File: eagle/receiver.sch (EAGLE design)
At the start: 20 parts, among them IC1 7805T, U1 ARDUINOR3-DIMENSION

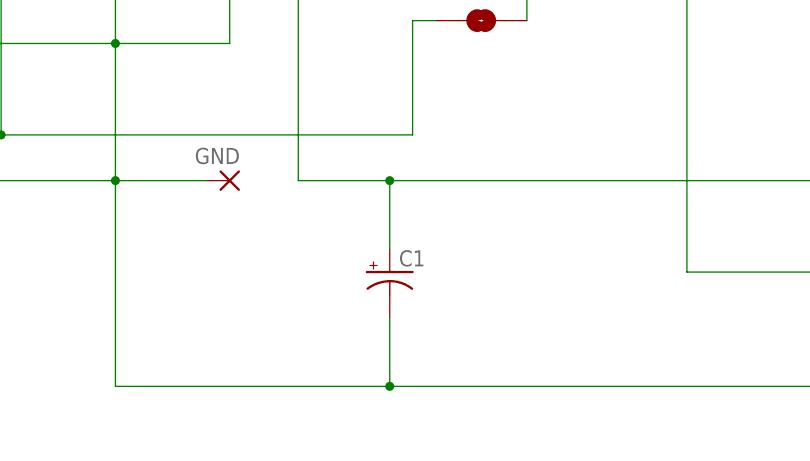
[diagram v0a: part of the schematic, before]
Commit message: Docs++
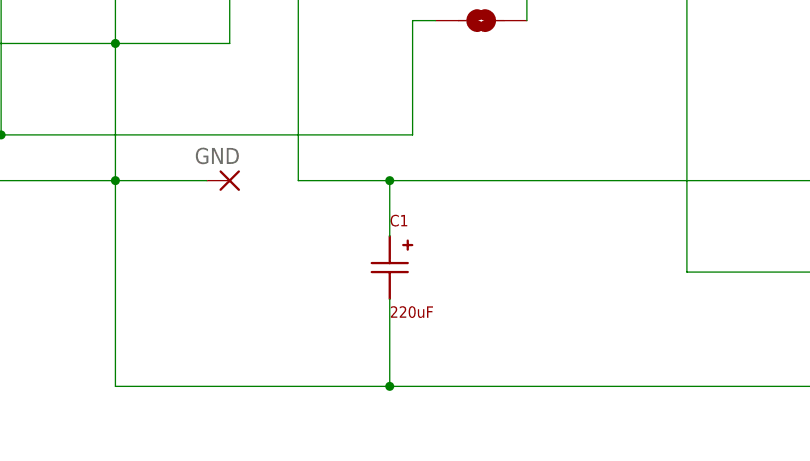
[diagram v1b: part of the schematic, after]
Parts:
- C1: value (none) -> 220uF; device adafruit:CPOL-US153CLV-0405 -> phrobo:UWT0J221MCL1GB
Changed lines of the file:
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@@
 <part name="RESET" library="SparkFun" deviceset="TAC_SWITCH" device="SMD"/>
 <part name="JP7" library="SparkFun" deviceset="M02" device="PTH"/>
-<part name="C1" library="adafruit" deviceset="CPOL-US" device="153CLV-0405"/>
+<part name="C1" library="phrobo" deviceset="UWT0J221MCL1GB" device="" value="220uF"/>
 <part name="D1" library="adafruit" deviceset="DIODE" device="SMA"/>
 <part name="VCC/+5V" library="SparkFun" deviceset="SOLDERJUMPER" device="NO" value="NC=+5v"/>
@@
 <junction x="45.72" y="86.36"/>
 <pinref part="C1" gate="G$1" pin="-"/>
-<wire x1="63.5" y1="20.32" x2="63.5" y2="12.7" width="0.1524" layer="91"/>
+<wire x1="63.5" y1="22.4" x2="63.5" y2="12.7" width="0.1524" layer="91"/>
 <junction x="63.5" y="12.7"/>
 </segment>
@@
 <wire x1="53.34" y1="88.9" x2="101.6" y2="88.9" width="0.1524" layer="91"/>
 <pinref part="C1" gate="G$1" pin="+"/>
-<wire x1="63.5" y1="27.94" x2="63.5" y2="35.56" width="0.1524" layer="91"/>
+<wire x1="63.5" y1="29.4" x2="63.5" y2="35.56" width="0.1524" layer="91"/>
 <junction x="63.5" y="35.56"/>
 <pinref part="+5V" gate="G$1" pin="VCC"/>
